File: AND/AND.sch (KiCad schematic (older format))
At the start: 8 parts, among them J1 Conn_01x08_Male, J2 Conn_01x08_Male, J3 Conn_01x08_Male, J4 Conn_01x04_Male, U1 74LS08, U2 74LS08, U3 74LS573

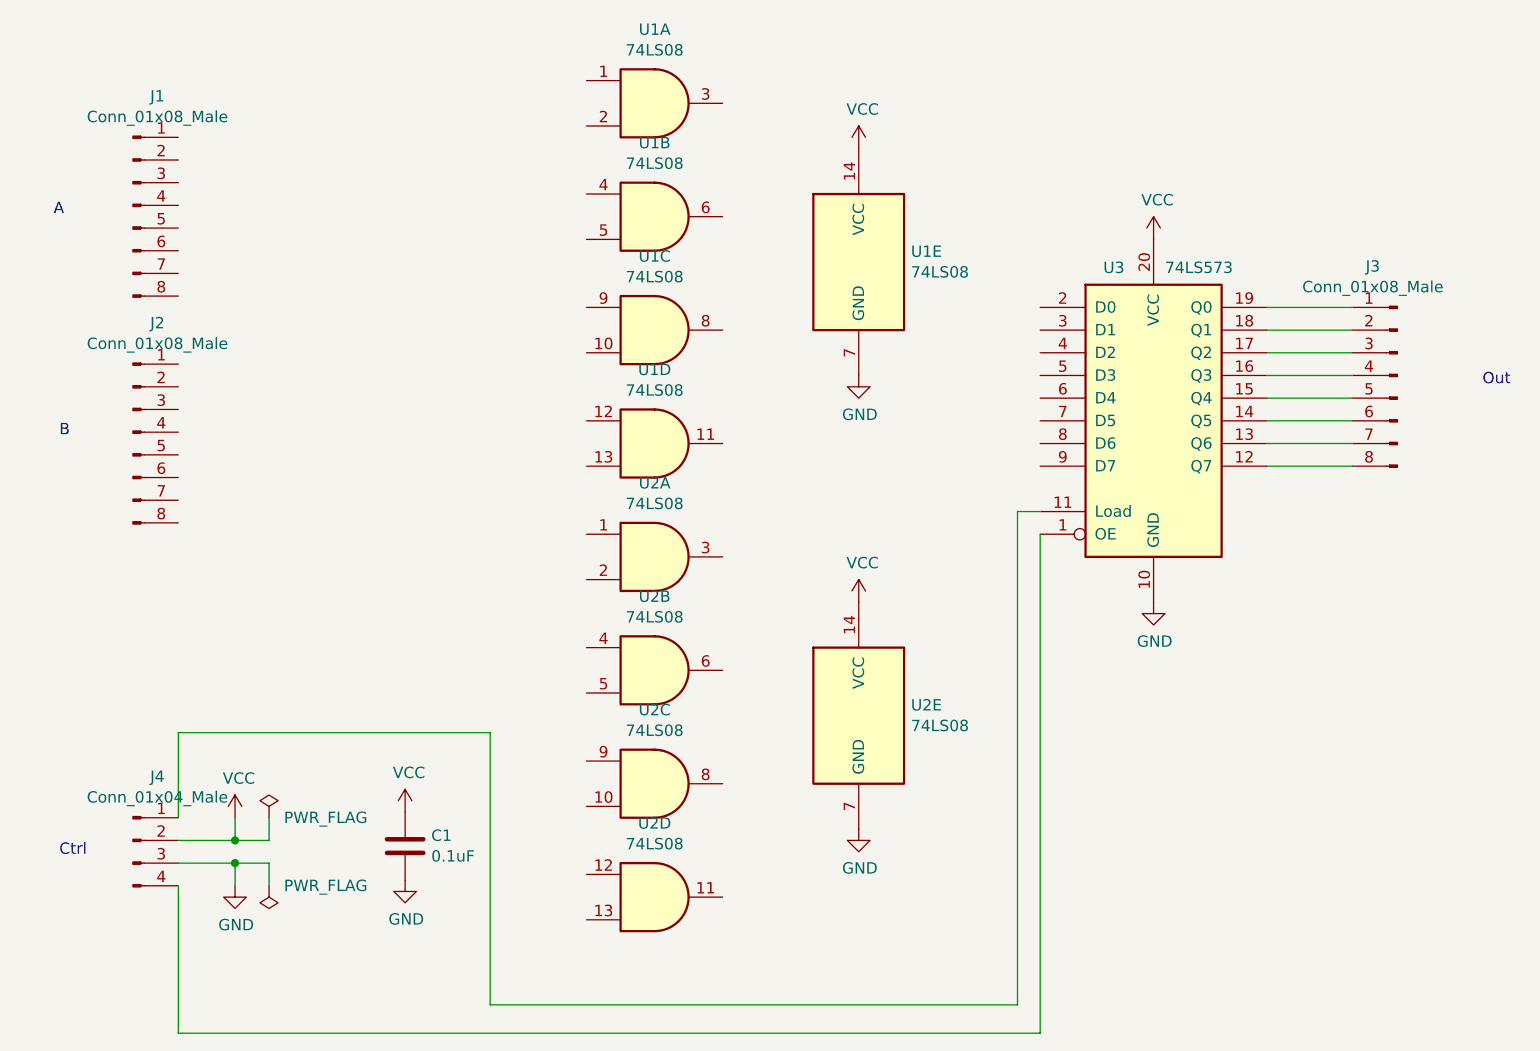
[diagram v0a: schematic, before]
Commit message: New template + 74HC573
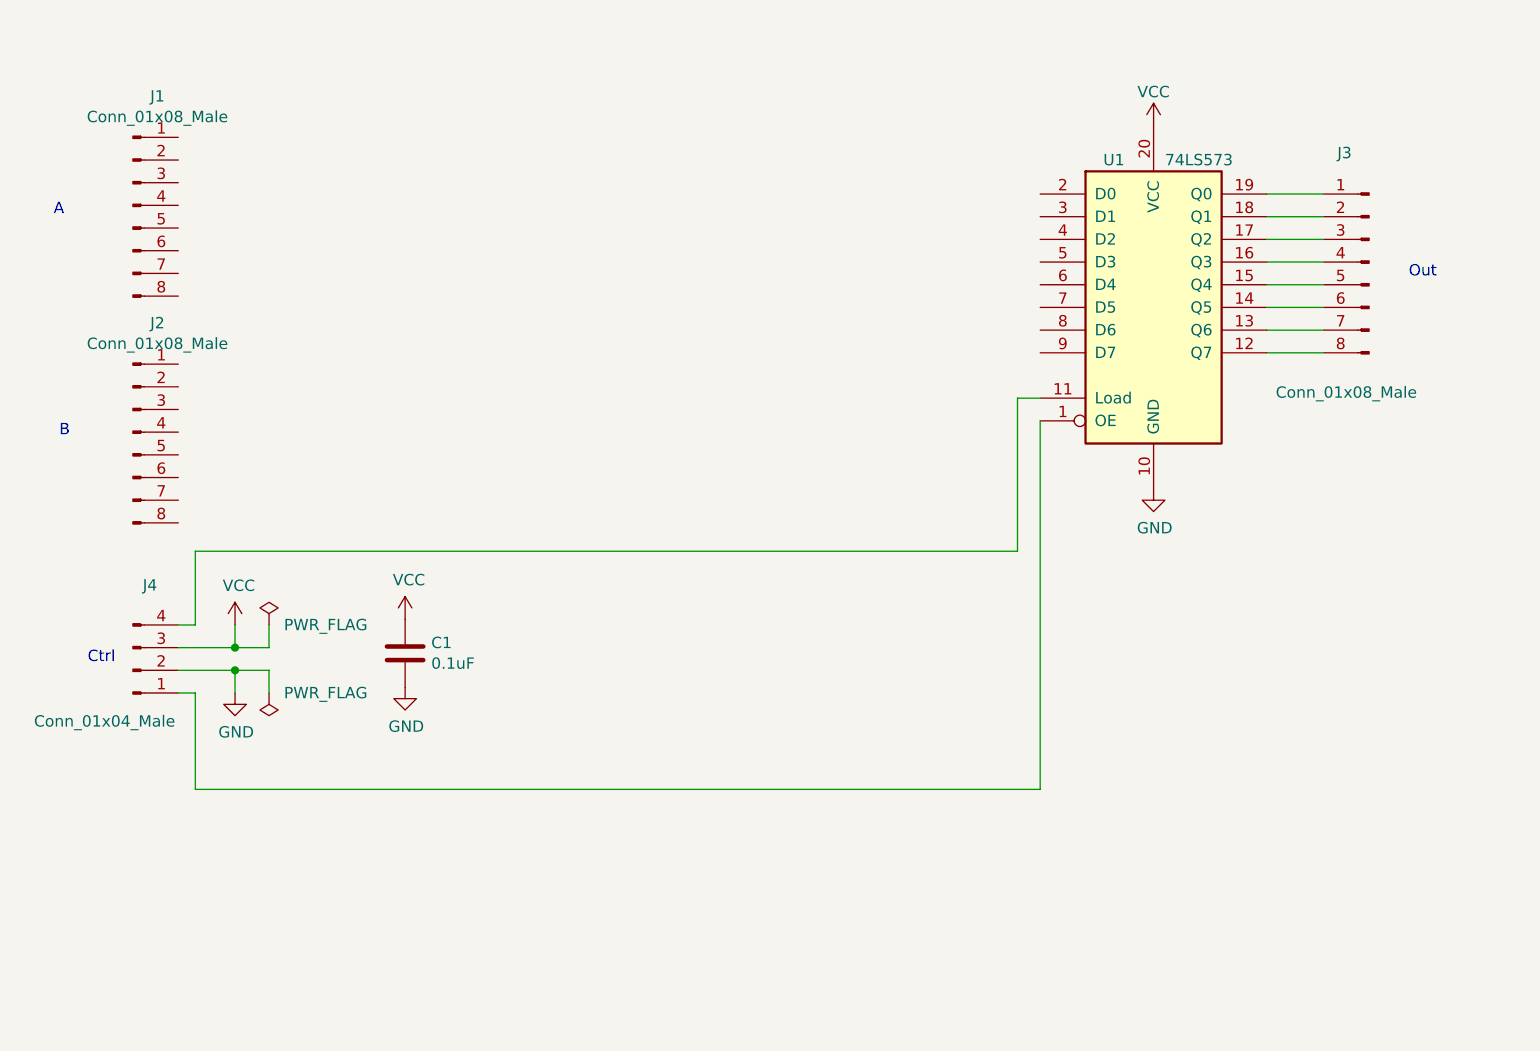
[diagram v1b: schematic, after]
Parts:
- removed U1, U2: 74LS08, Package_DIP:DIP-14_W7.62mm, symbol 74xx:74LS08
- removed U3: 74LS573, Package_DIP:DIP-20_W7.62mm, symbol 74xx:74LS573
- added U1: 74LS573, Package_DIP:DIP-20_W7.62mm, symbol 74xx:74LS573
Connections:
- net GND: now also J4.2 (Pin_2), U1.10 (GND); no longer J4.3 (Pin_3)
- net VCC: now also J4.3 (Pin_3), U1.20 (VCC); no longer J4.2 (Pin_2)
- net at J3.1 (Pin_1): now also U1.19 (Q0)
- net at J3.2 (Pin_2): now also U1.18 (Q1)
- net at J3.3 (Pin_3): now also U1.17 (Q2)
- net at J3.4 (Pin_4): now also U1.16 (Q3)
- net at J3.5 (Pin_5): now also U1.15 (Q4)
- net at J3.6 (Pin_6): now also U1.14 (Q5)
- net at J3.7 (Pin_7): now also U1.13 (Q6)
- net at J3.8 (Pin_8): now also U1.12 (Q7)
- net at J4.1 (Pin_1): now also U1.1 (OE)
- net at J4.4 (Pin_4): now also U1.11 (Load)
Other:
- moved on the sheet: C1, J3, J4
